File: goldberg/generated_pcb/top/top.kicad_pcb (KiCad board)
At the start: 2 copper layers, 116 x 115.3 mm, 0 parts

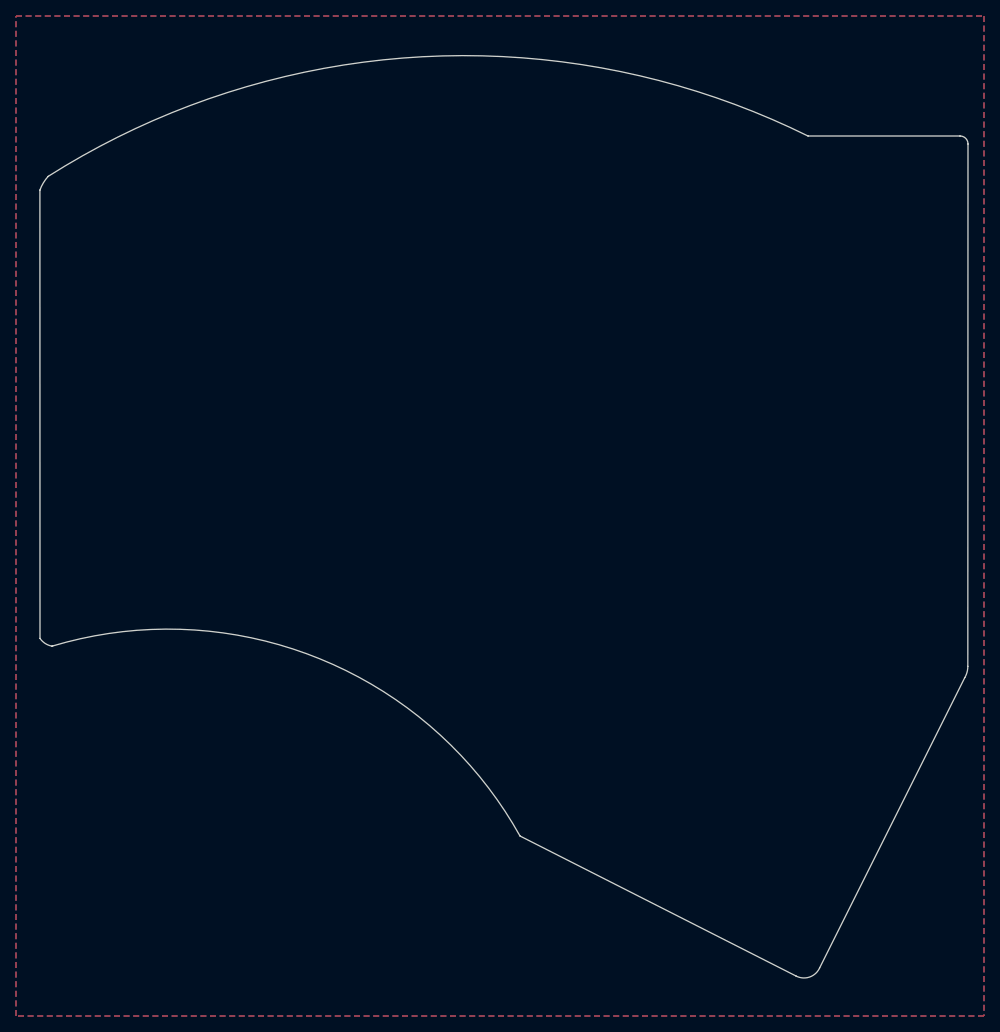
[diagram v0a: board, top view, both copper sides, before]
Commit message: PC change
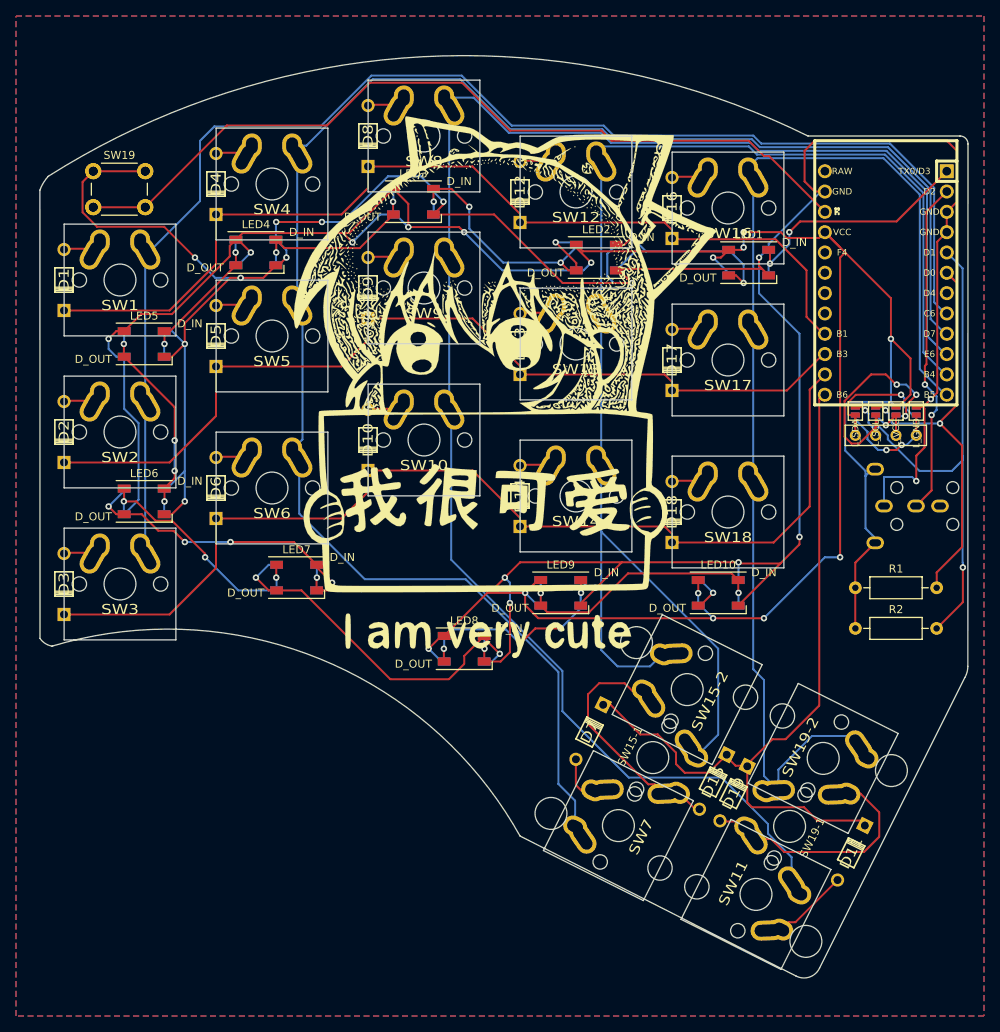
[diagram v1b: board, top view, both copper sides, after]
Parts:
- added D1: D, footprints:diode, F.Cu at (23.0, 39.0)
- added D10: D, footprints:diode, F.Cu at (61.0, 59.0)
- added D11: D, footprints:diode, F.Cu at (121.4, 110.6)
- added D12: D, footprints:diode, F.Cu at (80.0, 28.0)
- added D13: D, footprints:diode, F.Cu at (80.0, 47.0)
- added D14: D, footprints:diode, F.Cu at (80.0, 66.0)
- added D15: D, footprints:diode, F.Cu at (104.1, 101.7)
- added D16: D, footprints:diode, F.Cu at (99.0, 30.0)
- added D17: D, footprints:diode, F.Cu at (99.0, 49.0)
- added D18: D, footprints:diode, F.Cu at (99.0, 68.0)
- added D19: D, footprints:diode, F.Cu at (106.7, 103.2)
- added D2: D, footprints:diode, F.Cu at (23.0, 58.0)
- added D3: D, footprints:diode, F.Cu at (23.0, 77.0)
- added D4: D, footprints:diode, F.Cu at (42.0, 27.0)
- added D5: D, footprints:diode, F.Cu at (42.0, 46.0)
- added D6: D, footprints:diode, F.Cu at (42.0, 65.0)
- added D7: D, footprints:diode, F.Cu at (88.7, 95.5)
- added D8: D, footprints:diode, F.Cu at (61.0, 21.0)
- added D9: D, footprints:diode, F.Cu at (61.0, 40.0)
- added G***: LOGO, footprints:mokou-cute, F.Cu at (77.5, 52.1)
- added JP1: L_GND, footprints:Jumper, F.Cu at (129.5, 55.4)
- added JP2: L_VCC, footprints:Jumper, F.Cu at (127.0, 55.4)
- added JP3: L_SCL, footprints:Jumper, F.Cu at (124.5, 55.4)
- added JP4: L_SDA, footprints:Jumper, F.Cu at (121.9, 55.4)
- added JP5: R_GND, footprints:Jumper, B.Cu at (129.5, 55.4)
- added JP6: R_VCC, footprints:Jumper, B.Cu at (127.0, 55.4)
- added JP7: R_SCL, footprints:Jumper, B.Cu at (124.5, 55.4)
- added JP8: R_SDA, footprints:Jumper, B.Cu at (121.9, 55.4)
- added LED1: WS2812B, footprints:LED_WS2812B_4Pad, F.Cu at (108.6, 36.8)
- added LED10: WS2812B, footprints:LED_WS2812B_4Pad, F.Cu at (104.8, 78.1)
- added LED2: WS2812B, footprints:LED_WS2812B_4Pad, F.Cu at (89.5, 36.2)
- added LED3: WS2812B, footprints:LED_WS2812B_4Pad, F.Cu at (66.7, 29.2)
- added LED4: WS2812B, footprints:LED_WS2812B_4Pad, F.Cu at (47.0, 35.6)
- added LED5: WS2812B, footprints:LED_WS2812B_4Pad, F.Cu at (33.0, 47.0)
- added LED6: WS2812B, footprints:LED_WS2812B_4Pad, F.Cu at (33.0, 66.7)
- added LED7: WS2812B, footprints:LED_WS2812B_4Pad, F.Cu at (52.1, 76.2)
- added LED8: WS2812B, footprints:LED_WS2812B_4Pad, F.Cu at (73.0, 85.1)
- added LED9: WS2812B, footprints:LED_WS2812B_4Pad, F.Cu at (85.1, 78.1)
- added P1: OLED, footprints:SSD_1306_128x32, B.Cu at (129.5, 58.4)
- added R1: 4.7K, Resistor_THT:R_Axial_DIN0207_L6.3mm_D2.5mm_P10.16mm_Horizontal, F.Cu at (121.9, 77.5)
- added R2: 4.7K, Resistor_THT:R_Axial_DIN0207_L6.3mm_D2.5mm_P10.16mm_Horizontal, F.Cu at (121.9, 82.5)
- added SW1: switch, footprints:1u-dual, F.Cu at (30.0, 39.0)
- added SW10: switch, footprints:1u-dual, F.Cu at (68.0, 59.0)
- added SW11: switch, footprints:1u-dual, F.Cu at (109.5, 115.8)
- added SW12: switch, footprints:1u-dual, F.Cu at (87.0, 28.0)
- added SW13: switch, footprints:1u-dual, F.Cu at (87.0, 47.0)
- added SW14: switch, footprints:1u-dual, F.Cu at (87.0, 66.0)
- added SW15: SW_Push, Button_Switch_THT:SW_PUSH_6mm_H5mm, B.Cu at (33.1, 25.4)
- added SW15-1: switch, footprints:2u-dual, F.Cu at (96.6, 98.7)
- added SW15-2: switch, footprints:1u-dual, F.Cu at (100.9, 90.2)
- added SW16: switch, footprints:1u-dual, F.Cu at (106.0, 30.0)
- added SW17: switch, footprints:1u-dual, F.Cu at (106.0, 49.0)
- added SW18: switch, footprints:1u-dual, F.Cu at (106.0, 68.0)
- added SW19: SW_Push, Button_Switch_THT:SW_PUSH_6mm_H5mm, F.Cu at (26.7, 25.4)
- added SW19-1: switch, footprints:2u-dual, F.Cu at (113.7, 107.3)
- added SW19-2: switch, footprints:1u-dual, F.Cu at (117.9, 98.8)
- added SW2: switch, footprints:1u-dual, F.Cu at (30.0, 58.0)
- added SW3: switch, footprints:1u-dual, F.Cu at (30.0, 77.0)
- added SW4: switch, footprints:1u-dual, F.Cu at (49.0, 27.0)
- added SW5: switch, footprints:1u-dual, F.Cu at (49.0, 46.0)
- added SW6: switch, footprints:1u-dual, F.Cu at (49.0, 65.0)
- added SW7: switch, footprints:1u-dual, F.Cu at (92.3, 107.2)
- added SW8: switch, footprints:1u-dual, F.Cu at (68.0, 21.0)
- added SW9: switch, footprints:1u-dual, F.Cu at (68.0, 40.0)
- added U1: TRRS, footprints:trrs, B.Cu at (135.7, 67.2)
- added U2: promicro-squiggle, footprints:promicro, B.Cu at (125.7, 39.4)
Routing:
- net GND: track 0.00 -> 412.4 mm, vias 0 -> 19
- net VCC: track 0.00 -> 378.1 mm, vias 0 -> 19
- net COL1: track 0.00 -> 209.7 mm
- net COL2: track 0.00 -> 204.9 mm
- net COL3: track 0.00 -> 171.2 mm
- net COL0: track 0.00 -> 169.3 mm
- net COL4: track 0.00 -> 139.3 mm
- net ROW2: track 0.00 -> 130.0 mm
- net ROW0: track 0.00 -> 120.9 mm
- net ROW1: track 0.00 -> 114.5 mm
- net Net-(SW15-Pad2): track 0.00 -> 104.6 mm
- net ROW3: track 0.00 -> 95.3 mm
- net SDA: track 0.00 -> 69.3 mm, vias 0 -> 2
- net SCL: track 0.00 -> 54.0 mm, vias 0 -> 2
- net Net-(LED7-Pad2): track 0.00 -> 45.3 mm, vias 0 -> 2
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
